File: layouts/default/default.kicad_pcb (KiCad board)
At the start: 2 copper layers, 50 x 35 mm, 22 parts

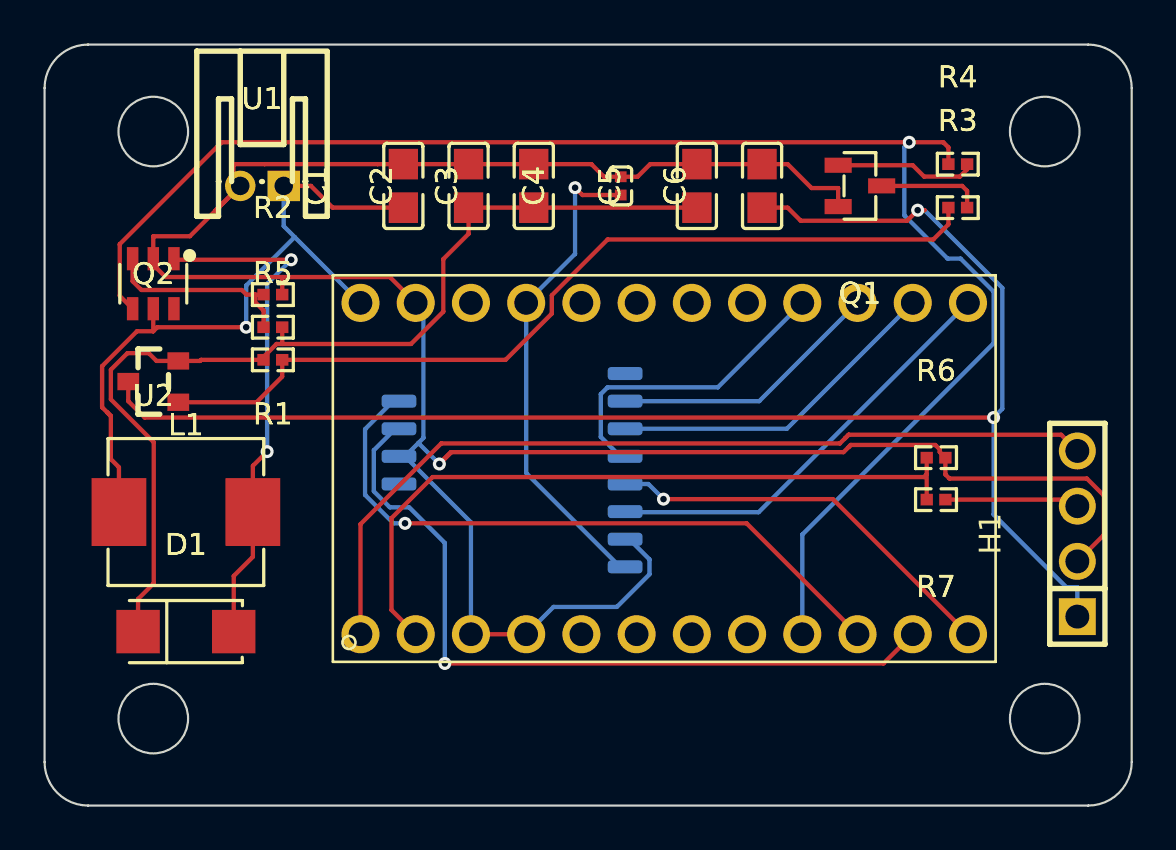
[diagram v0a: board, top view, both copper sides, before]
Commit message: Update PCB layout
Co-Authored-By: Claude Opus 4.5 <noreply@anthropic.com>
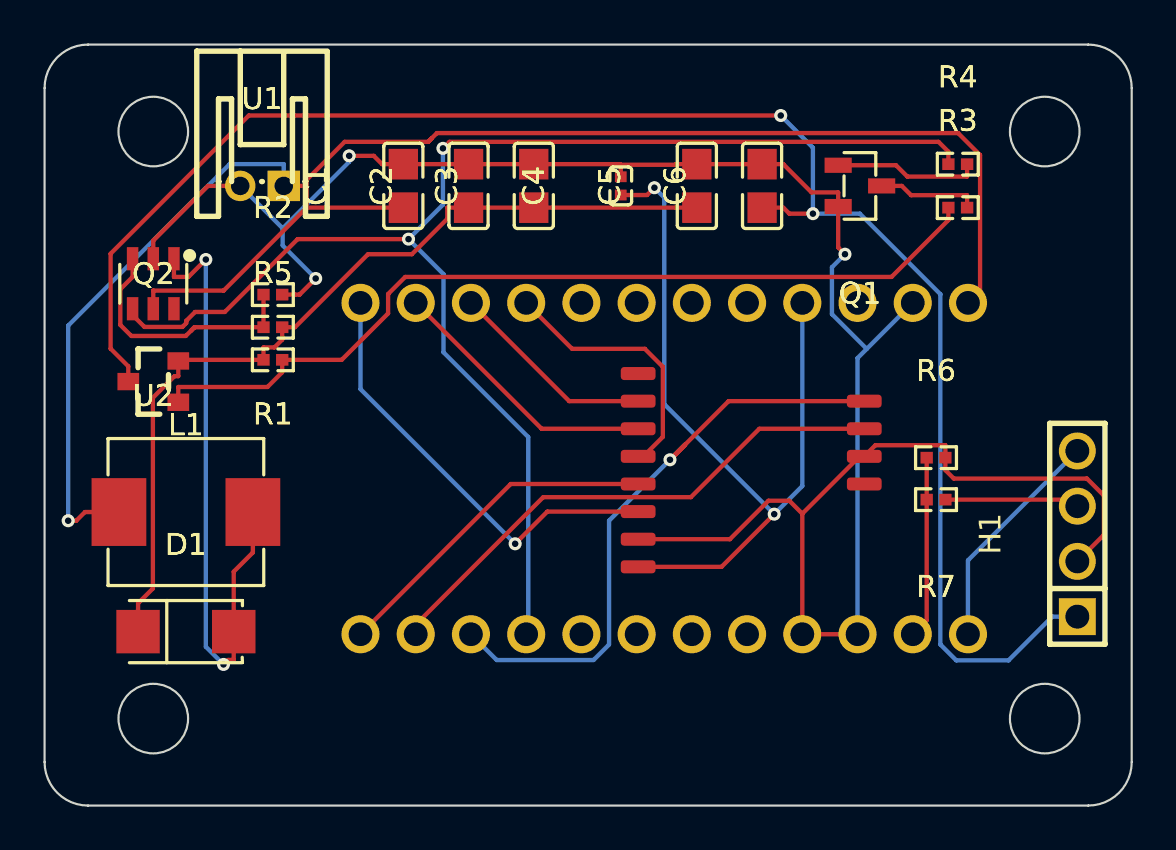
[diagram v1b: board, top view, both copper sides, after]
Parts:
- U3: moved to F.Cu
- U4: moved to B.Cu
- turned U4 to 180 degrees
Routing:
- net power_raw-VCC: track 33.5 -> 81.3 mm
- net TX: track 40.3 -> 10.5 mm
- net mcu-uart-RX: track 33.2 -> 8.39 mm
- net GND: track 119.7 -> 103.3 mm, vias 1 -> 3
- net power_gnd-VCC: track 22.6 -> 36.5 mm, vias 1 -> 2
- net busy: track 35.3 -> 24.8 mm, vias 1 -> 0
- net enable: track 72.6 -> 64.4 mm, vias 1 -> 2
- net power_out-VCC: track 72.4 -> 78.2 mm
- net A: track 23.6 -> 29.3 mm
- net power_in-VCC: track 46.5 -> 41.7 mm
- net footprint-reset-0: track 18.6 -> 15.6 mm, vias 1 -> 0
- net MOSI: track 15.6 -> 12.6 mm
- net MISO: track 12.6 -> 9.56 mm
- net FB: track 8.97 -> 12.0 mm
- net SCLK: track 14.5 -> 12.2 mm
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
